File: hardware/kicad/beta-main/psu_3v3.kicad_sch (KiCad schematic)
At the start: 0 parts

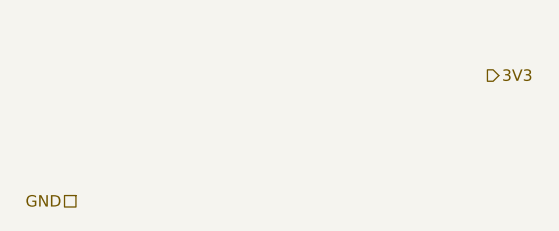
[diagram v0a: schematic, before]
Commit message: tweaks and added servo controller
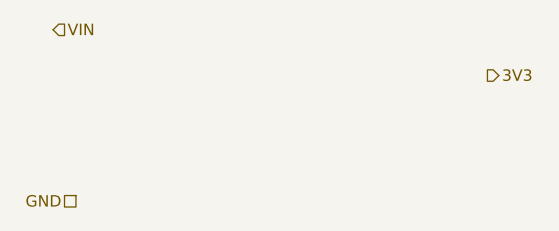
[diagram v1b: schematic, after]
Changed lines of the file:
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@@
 		(comment 1 "Powers: DISPLAY")
+	)
+	(hierarchical_label "VIN"
+		(shape input)
+		(at 55.88 43.18 0)
+		(effects
+			(font
+				(size 1.27 1.27)
+			)
+			(justify left)
+		)
 	)
 	(hierarchical_label "3V3"
